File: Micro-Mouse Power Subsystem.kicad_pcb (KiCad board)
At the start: 2 copper layers, 80 x 60 mm, 103 parts, among them J1 Pin Header, J2 TYPE-C-31-M-12, J3 Conn_01x02, Q1 2N7002, Q2 AO3401A, Q3 AO3400A, Q4 AO3400A, Q5 AO3401A, SW1 SW_SPDT, U1 TP4056-42-ESOP8, U2 brushed DC motors, U3 auxiliary motors, U4 HUSB237-AA001-DN06R, U5 TPS61088RHLR, U6 INA219AIDCNR, U7 XL1509-3.3, U8 XL1509-5.0

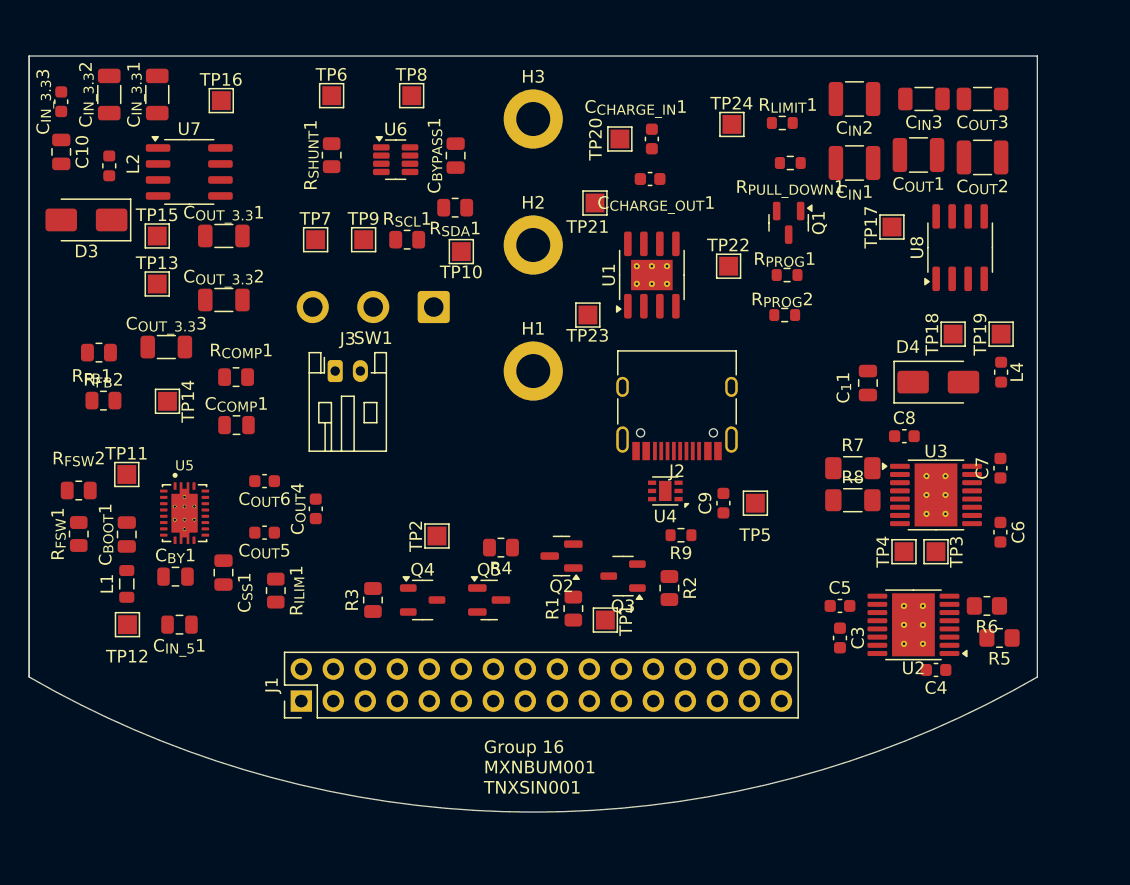
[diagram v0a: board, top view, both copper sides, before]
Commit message: updated pcb layout
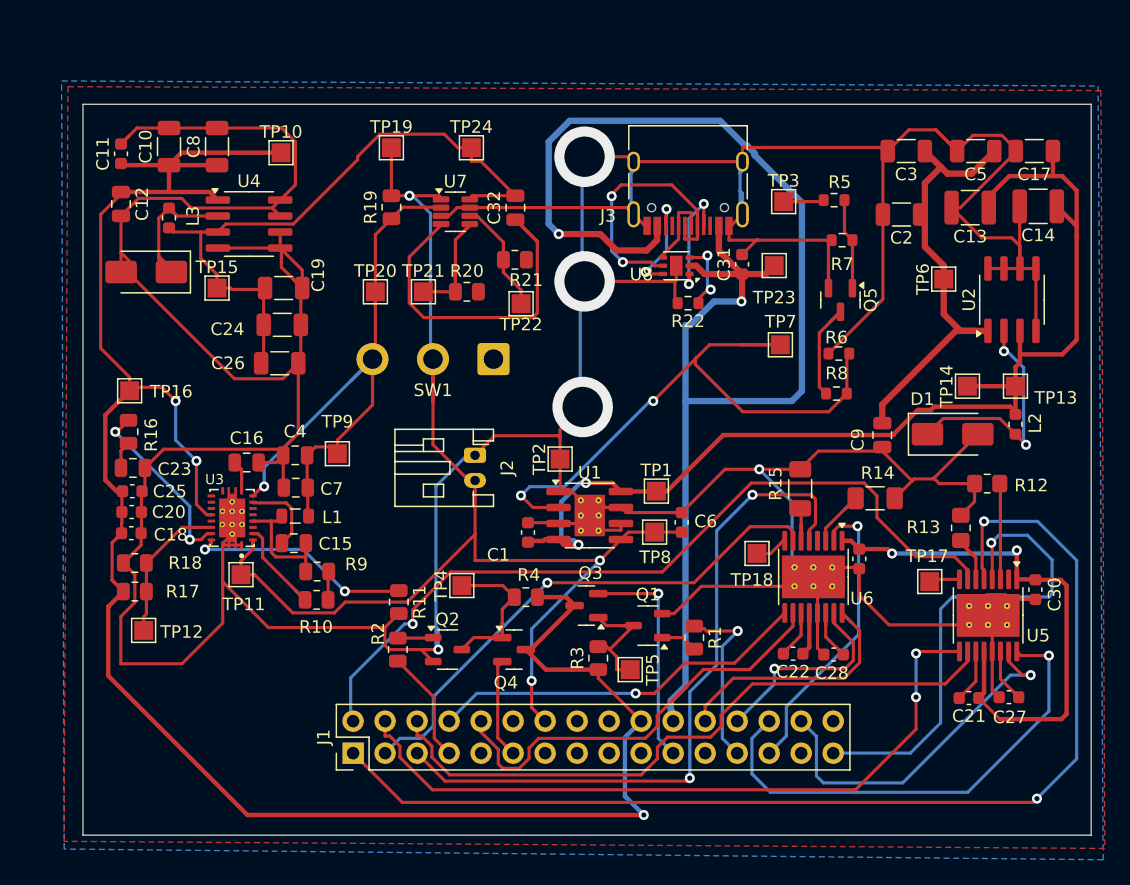
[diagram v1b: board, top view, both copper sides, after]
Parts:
- removed H1, H2, H3: MountingHole_2.7mm_M2.5_DIN965_Pad, MountingHole:MountingHole_2.7mm_M2.5_DIN965_Pad
- removed the TP20 at (139.7, 78.1)
- added TP1: 5V_BAT_CHRG, TestPoint:TestPoint_Pad_1.5x1.5mm, F.Cu at (142.6, 106.0)
- C2: renamed from C_{IN}1; footprint Capacitor_SMD:C_1210_3225Metric -> Capacitor_SMD:C_1206_3216Metric
- C3: renamed from C_{IN}2; footprint Capacitor_SMD:C_1210_3225Metric -> Capacitor_SMD:C_1206_3216Metric
- TP10: renamed from TP16; value 5V_REG2 -> 5V_OUT
- TP16: renamed from TP13; value 5V_REG -> 5V_VOUT
- moved C1 32.7 mm to (132.4, 109.3), turned to 90 degrees
- moved C6 27.4 mm to (144.6, 108.5), turned to 90 degrees
- moved TP8 26.5 mm to (142.5, 109.3), turned to 180 degrees
- moved TP9 21.5 mm to (117.3, 103.1), turned to 180 degrees
- moved R10 20.8 mm to (115.6, 114.7)
- moved C28 19.8 mm to (156.7, 119.0), turned to 0 degrees
- moved U1 19.7 mm to (137.3, 108.0), turned to 0 degrees
- moved R17 19.2 mm to (101.2, 114.0), turned to 180 degrees
- moved R9 19.2 mm to (115.7, 112.4), turned to 0 degrees
- moved C22 19.1 mm to (153.4, 119.0), turned to 180 degrees
- moved C31 19.0 mm to (149.4, 88.0)
- moved TP23 18.9 mm to (151.9, 88.2)
- moved R22 18.4 mm to (145.1, 91.1)
- moved TP12 18.3 mm to (101.9, 117.1), turned to 90 degrees
- moved J3 17.9 mm to (145.1, 81.0)
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- renumbered C_{CHARGE_IN}1 to C1, C_{IN_3.3}2 to C10, C_{IN_3.3}3 to C11, C10 to C12, C_{OUT}1 to C13, C_{OUT}2 to C14, C_{BOOT}1 to C15, C_{SS}1 to C16, C_{OUT}3 to C17, C_{OUT}4 to C18, C_{OUT_3.3}1 to C19, C_{OUT}5 to C20, C5 to C21, C6 to C22, C_{COMP}1 to C23, C_{OUT_3.3}2 to C24, C_{OUT}6 to C25, C_{OUT_3.3}3 to C26, C3 to C27, C7 to C28, C8 to C29, C4 to C30, C9 to C31, C_{BYPASS}1 to C32, C_{BY}1 to C4, C_{IN}3 to C5, C_{CHARGE_OUT}1 to C6, C_{IN_5}1 to C7, C_{IN_3.3}1 to C8, C_{1}1 to C9, D4 to D1, D3 to D2, J3 to J2, J2 to J3, L4 to L2, L2 to L3, Q3 to Q1, Q4 to Q2, Q2 to Q3, Q5 to Q4, Q1 to Q5, R2 to R1, R_{FSW}2 to R10, R_{ILIM}1 to R11, R5 to R12, R6 to R13, R7 to R14, R8 to R15, R_{COMP}1 to R16, R_{FB}1 to R17, R_{FB}2 to R18, R_{SHUNT}1 to R19, R3 to R2, R_{SCL}1 to R20, R_{SDA}1 to R21, R9 to R22, R1 to R3, R_{LIMIT}1 to R5, R_{PROG}1 to R6, R_{PULL_DOWN}1 to R7, R_{PROG}2 to R8, R_{FSW}1 to R9, TP14 to TP12, TP19 to TP13, TP18 to TP14, TP3 to TP17, TP4 to TP18, TP6 to TP19, TP23 to TP2, TP7 to TP20, TP9 to TP21, TP10 to TP22, TP5 to TP23, TP8 to TP24, TP24 to TP3, TP2 to TP4, TP1 to TP5, TP17 to TP6, TP22 to TP7, TP21 to TP8, TP12 to TP9, U8 to U2, U5 to U3, U7 to U4, U2 to U5, U3 to U6, U6 to U7, U4 to U8
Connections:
- J1 pad 1: /Motor2_B_OUT -> /MOTOR2_B_OUT
- J1 pad 14: /Battery  -> /BATTERY
- J1 pad 2: /Motor2_A_OUT -> /MOTOR2_A_OUT
- J1 pad 20: /5V Out  -> /5V_OUT
- J1 pad 3: /Motor4_A_OUT -> /MOTOR4_A_OUT
- J1 pad 5: /Motor4_B_OUT -> /MOTOR4_B_OUT
- Q3 pad 3: /5V Out  -> /5V_OUT
- Q4 pad 3: /5V Out  -> /5V_OUT
- R3 pad 1: /5V Out  -> /5V_OUT
- R4 pad 1: /5V Out  -> /5V_OUT
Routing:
- net GND: track 0.00 -> 514.2 mm, vias 0 -> 5
- net /5V_OUT: track 0.00 -> 166.2 mm, vias 0 -> 3
- net /HV (9V): track 0.00 -> 119.0 mm, vias 0 -> 2
- net /BATTERY: track 0.00 -> 104.2 mm, vias 0 -> 3
- net /5V_BAT_CHARGE: track 0.00 -> 90.9 mm, vias 0 -> 2
- net /MOTOR2_B_OUT: track 0.00 -> 89.6 mm, vias 0 -> 2
- net /MOTOR2_A_OUT: track 0.00 -> 63.7 mm, vias 0 -> 1
- net /MOTOR2_CTRL1: track 0.00 -> 57.7 mm, vias 0 -> 2
- net /MOTOR4_B_OUT: track 0.00 -> 56.3 mm, vias 0 -> 2
- net /SWITCH_OUT: track 0.00 -> 53.7 mm, vias 0 -> 1
- net /3.3V_OUT: track 0.00 -> 53.0 mm
- net /MOTOR2_CTRL2: track 0.00 -> 52.8 mm
- net Net-(U1-PROG): track 0.00 -> 50.6 mm, vias 0 -> 2
- net /5V Out : track 0.00 -> 47.4 mm, vias 0 -> 2
- net /MOTOR4_A_OUT: track 0.00 -> 42.4 mm, vias 0 -> 1
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- added copper zone on F.Cu, net (none)
- added copper zone on B.Cu, net GND
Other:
- board size 80 x 60 mm -> 80 x 58 mm
